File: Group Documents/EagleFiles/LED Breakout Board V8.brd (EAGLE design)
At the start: 31.4 x 45.5 mm, 6 parts

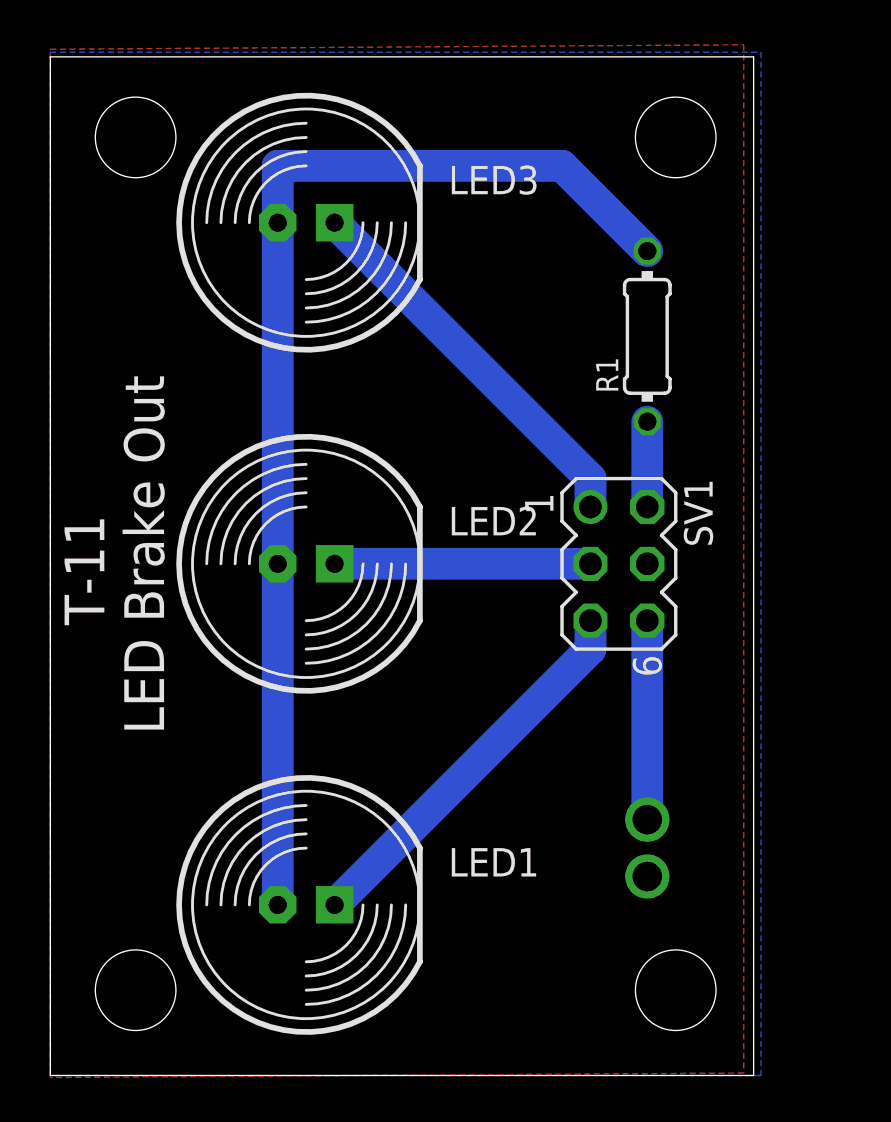
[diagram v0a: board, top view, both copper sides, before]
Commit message: LED BOB
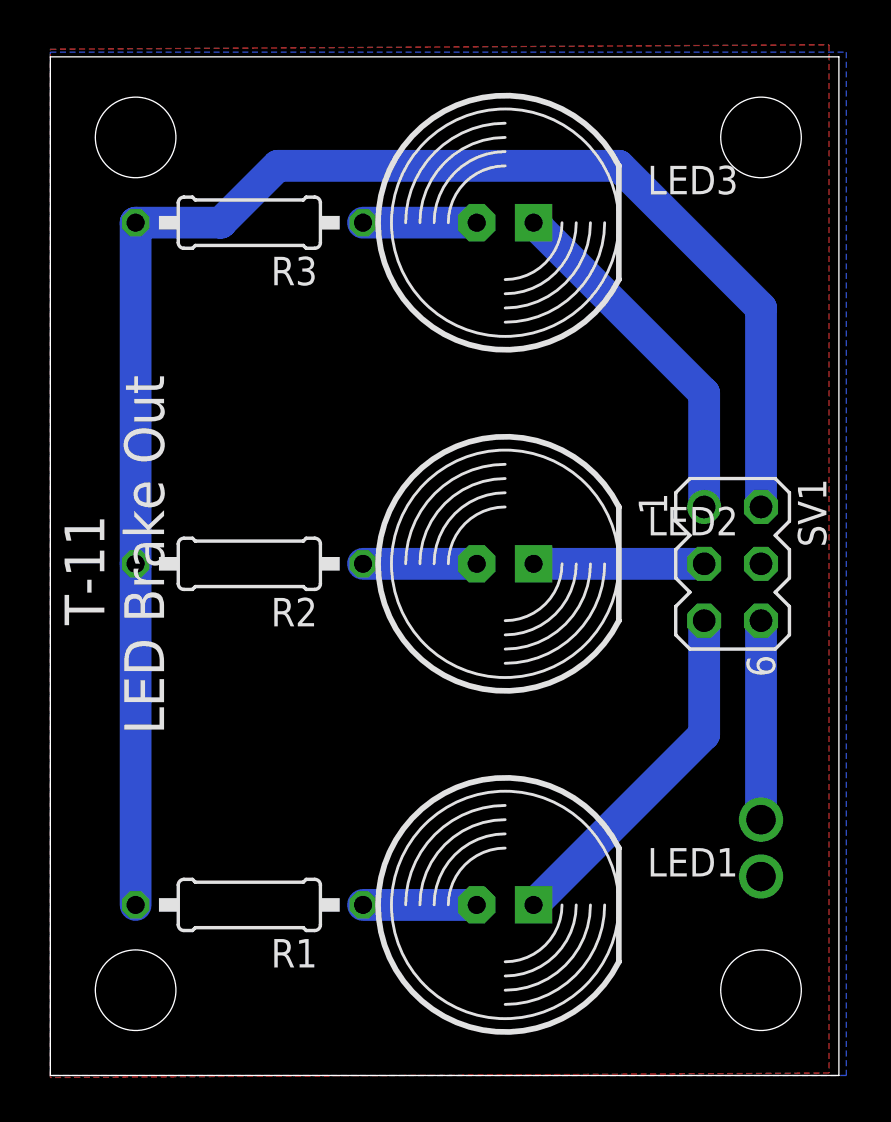
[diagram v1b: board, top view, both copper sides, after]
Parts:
- added R2, R3: 330, eagle-ltspice:0207/10
- R1: device eagle-ltspice:0204/7 -> eagle-ltspice:0207/10
- moved R1 31.0 mm to (8.89, 7.62), turned to 180 degrees
- moved LED1 8.89 mm to (20.3, 7.62)
- moved LED2 8.89 mm to (20.3, 22.9)
- moved LED3 8.89 mm to (20.3, 38.1)
- moved SV1 5.08 mm to (30.5, 22.9)
- moved SW 5.08 mm to (31.8, 10.2)
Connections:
- removed net N$1: LED1.A, LED2.A, LED3.A, R1.2
- new net N$2: LED3.A, R3.1
- new net N$3: LED2.A, R2.1
- new net N$4: LED1.A, R1.1
- net +5V: now also R1.2, R2.2, R3.2; no longer R1.1
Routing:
- net +5V: track 3.81 -> 71.0 mm
- net N$1: track 51.1 -> 0.00 mm
- net N$4: track 0.00 -> 5.08 mm
- net N$3: track 0.00 -> 5.08 mm
- net N$2: track 0.00 -> 5.08 mm
- net PD1: track 11.4 -> 7.62 mm
- net PD2: track 17.4 -> 15.9 mm
- net PD0: track 17.4 -> 15.9 mm
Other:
- board size 31.4 x 45.5 mm -> 35.2 x 45.5 mm
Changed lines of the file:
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@@
 <board>
 <plain>
-<wire x1="0" y1="0" x2="31.42" y2="0" width="0" layer="20"/>
-<wire x1="31.42" y1="0" x2="31.42" y2="45.51" width="0" layer="20"/>
-<wire x1="31.42" y1="45.51" x2="0" y2="45.51" width="0" layer="20"/>
+<wire x1="0" y1="0" x2="35.23" y2="0" width="0" layer="20"/>
+<wire x1="35.23" y1="0" x2="35.23" y2="45.51" width="0" layer="20"/>
+<wire x1="35.23" y1="45.51" x2="0" y2="45.51" width="0" layer="20"/>
 <wire x1="0" y1="45.51" x2="0" y2="0" width="0" layer="20"/>
 <text x="5.08" y="15.24" size="1.778" layer="25" rot="R90">       T-11
 LED Brake Out</text>
 <hole x="3.81" y="41.91" drill="3.6"/>
-<hole x="27.94" y="41.91" drill="3.6"/>
-<hole x="27.94" y="3.81" drill="3.6"/>
+<hole x="31.75" y="41.91" drill="3.6"/>
+<hole x="31.75" y="3.81" drill="3.6"/>
 <hole x="3.81" y="3.81" drill="3.6"/>
 </plain>
@@
 </autorouter>
 <elements>
-<element name="SV1" library="con-lstb" package="MA03-2" value="" x="25.4" y="22.86" rot="R270">
-<attribute name="OC_NEWARK" value="unknown" x="25.4" y="22.86" size="1.778" layer="27" rot="R270" display="off"/>
-<attribute name="MPN" value="" x="25.4" y="22.86" size="1.778" layer="27" rot="R270" display="off"/>
-<attribute name="MF" value="" x="25.4" y="22.86" size="1.778" layer="27" rot="R270" display="off"/>
-<attribute name="OC_FARNELL" value="unknown" x="25.4" y="22.86" size="1.778" layer="27" rot="R270" display="off"/>
-</element>
-<element name="SW" library="pushbutton" package="PUSHBUTTON" value="PUSHBUTTON" x="26.67" y="10.16" rot="R90"/>
-<element name="LED1" library="led" package="LED10MM" value="" x="11.43" y="7.62"/>
-<element name="LED2" library="led" package="LED10MM" value="" x="11.43" y="22.86"/>
-<element name="LED3" library="led" package="LED10MM" value="" x="11.43" y="38.1"/>
-<element name="R1" library="eagle-ltspice" package="0204/7" value="330" x="26.67" y="33.02" rot="R90">
-<attribute name="SPICEMODEL" value="NONE" x="26.67" y="33.02" size="1.778" layer="27" rot="R90" display="off"/>
-<attribute name="SPICEPREFIX" value="R" x="26.67" y="33.02" size="1.778" layer="27" rot="R90" display="off"/>
+<element name="SV1" library="con-lstb" package="MA03-2" value="" x="30.48" y="22.86" rot="R270">
+<attribute name="OC_NEWARK" value="unknown" x="30.48" y="22.86" size="1.778" layer="27" rot="R270" display="off"/>
+<attribute name="MPN" value="" x="30.48" y="22.86" size="1.778" layer="27" rot="R270" display="off"/>
+<attribute name="MF" value="" x="30.48" y="22.86" size="1.778" layer="27" rot="R270" display="off"/>
+<attribute name="OC_FARNELL" value="unknown" x="30.48" y="22.86" size="1.778" layer="27" rot="R270" display="off"/>
+</element>
+<element name="SW" library="pushbutton" package="PUSHBUTTON" value="PUSHBUTTON" x="31.75" y="10.16" rot="R90"/>
+<element name="LED1" library="led" package="LED10MM" value="" x="20.32" y="7.62"/>
+<element name="LED2" library="led" package="LED10MM" value="" x="20.32" y="22.86"/>
+<element name="LED3" library="led" package="LED10MM" value="" x="20.32" y="38.1"/>
+<element name="R2" library="eagle-ltspice" package="0207/10" value="330" x="8.89" y="22.86" rot="R180">
+<attribute name="SPICEMODEL" value="NONE" x="8.89" y="22.86" size="1.778" layer="27" rot="R180" display="off"/>
+<attribute name="SPICEPREFIX" value="R" x="8.89" y="22.86" size="1.778" layer="27" rot="R180" display="off"/>
+</element>
+<element name="R3" library="eagle-ltspice" package="0207/10" value="330" x="8.89" y="38.1" rot="R180">
+<attribute name="SPICEMODEL" value="NONE" x="8.89" y="38.1" size="1.778" layer="27" rot="R180" display="off"/>
+<attribute name="SPICEPREFIX" value="R" x="8.89" y="38.1" size="1.778" layer="27" rot="R180" display="off"/>
+</element>
+<element name="R1" library="eagle-ltspice" package="0207/10" value="330" x="8.89" y="7.62" rot="R180">
+<attribute name="SPICEMODEL" value="NONE" x="8.89" y="7.62" size="1.778" layer="27" rot="R180" display="off"/>
+<attribute name="SPICEPREFIX" value="R" x="8.89" y="7.62" size="1.778" layer="27" rot="R180" display="off"/>
 </element>
 </elements>
@@
 <contactref element="SW" pad="OUT"/>
 <contactref element="SV1" pad="6"/>
-<wire x1="26.67" y1="11.43" x2="26.67" y2="20.32" width="1.4224" layer="16"/>
+<wire x1="31.75" y1="20.32" x2="31.75" y2="11.43" width="1.4224" layer="16"/>
 </signal>
 <signal name="PD1">
 <contactref element="SV1" pad="3"/>
 <contactref element="LED2" pad="K"/>
-<wire x1="12.7" y1="22.86" x2="24.13" y2="22.86" width="1.4224" layer="16"/>
+<wire x1="21.59" y1="22.86" x2="29.21" y2="22.86" width="1.4224" layer="16"/>
 </signal>
 <signal name="PD0">
 <contactref element="SV1" pad="5"/>
 <contactref element="LED1" pad="K"/>
-<wire x1="12.7" y1="7.62" x2="24.13" y2="19.05" width="1.4224" layer="16"/>
-<wire x1="24.13" y1="19.05" x2="24.13" y2="20.32" width="1.4224" layer="16"/>
+<wire x1="29.21" y1="20.32" x2="29.21" y2="15.24" width="1.4224" layer="16"/>
+<wire x1="29.21" y1="15.24" x2="21.59" y2="7.62" width="1.4224" layer="16"/>
 </signal>
 <signal name="PD2">
 <contactref element="SV1" pad="1"/>
 <contactref element="LED3" pad="K"/>
-<wire x1="12.7" y1="38.1" x2="24.13" y2="26.67" width="1.4224" layer="16"/>
-<wire x1="24.13" y1="26.67" x2="24.13" y2="25.4" width="1.4224" layer="16"/>
+<wire x1="29.21" y1="25.4" x2="29.21" y2="30.48" width="1.4224" layer="16"/>
+<wire x1="29.21" y1="30.48" x2="21.59" y2="38.1" width="1.4224" layer="16"/>
 </signal>
 <signal name="GND">
@@
 <polygon width="0.6096" layer="1" isolate="0.3048">
 <vertex x="0" y="45.85"/>
-<vertex x="30.98" y="46.05"/>
-<vertex x="30.98" y="0.11"/>
+<vertex x="34.79" y="46.05"/>
+<vertex x="34.79" y="0.11"/>
 <vertex x="0" y="-0.09"/>
 </polygon>
 <polygon width="0.4064" layer="16" isolate="0.3048">
 <vertex x="0" y="45.72"/>
-<vertex x="31.75" y="45.72"/>
-<vertex x="31.75" y="0"/>
+<vertex x="35.56" y="45.72"/>
+<vertex x="35.56" y="0"/>
 <vertex x="0" y="0"/>
 </polygon>
@@
 <signal name="+5V">
 <contactref element="SV1" pad="2"/>
+<contactref element="R3" pad="2"/>
+<contactref element="R1" pad="2"/>
+<contactref element="R2" pad="2"/>
+<wire x1="31.75" y1="25.4" x2="31.75" y2="34.29" width="1.4224" layer="16"/>
+<wire x1="31.75" y1="34.29" x2="25.4" y2="40.64" width="1.4224" layer="16"/>
+<wire x1="3.81" y1="38.1" x2="7.62" y2="38.1" width="1.4224" layer="16"/>
+<wire x1="7.62" y1="38.1" x2="10.16" y2="40.64" width="1.4224" layer="16"/>
+<wire x1="10.16" y1="40.64" x2="25.4" y2="40.64" width="1.4224" layer="16"/>
+<wire x1="3.81" y1="38.1" x2="3.81" y2="22.86" width="1.4224" layer="16"/>
+<wire x1="3.81" y1="22.86" x2="3.81" y2="7.62" width="1.4224" layer="16"/>
+</signal>
+<signal name="N$2">
+<contactref element="R3" pad="1"/>
+<contactref element="LED3" pad="A"/>
+<wire x1="19.05" y1="38.1" x2="13.97" y2="38.1" width="1.4224" layer="16"/>
+</signal>
+<signal name="N$3">
+<contactref element="R2" pad="1"/>
+<contactref element="LED2" pad="A"/>
+<wire x1="13.97" y1="22.86" x2="19.05" y2="22.86" width="1.4224" layer="16"/>
+</signal>
+<signal name="N$4">
 <contactref element="R1" pad="1"/>
-<wire x1="26.67" y1="29.21" x2="26.67" y2="25.4" width="1.4224" layer="16"/>
-</signal>
-<signal name="N$1">
 <contactref element="LED1" pad="A"/>
-<contactref element="LED2" pad="A"/>
-<contactref element="LED3" pad="A"/>
-<wire x1="22.86" y1="40.64" x2="10.16" y2="40.64" width="1.4224" layer="16"/>
-<wire x1="10.16" y1="40.64" x2="10.16" y2="38.1" width="1.4224" layer="16"/>
-<wire x1="10.16" y1="38.1" x2="10.16" y2="22.86" width="1.4224" layer="16"/>
-<wire x1="10.16" y1="22.86" x2="10.16" y2="7.62" width="1.4224" layer="16"/>
-<contactref element="R1" pad="2"/>
-<wire x1="22.86" y1="40.64" x2="26.67" y2="36.83" width="1.4224" layer="16"/>
+<wire x1="13.97" y1="7.62" x2="19.05" y2="7.62" width="1.4224" layer="16"/>
 </signal>
 </signals>
